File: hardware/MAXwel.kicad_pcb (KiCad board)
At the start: 2 copper layers, 85.1 x 87.2 mm, 155 parts, among them J1 Conn_02x05_Odd_Even, J2 Conn_02x12_Counter_Clockwise, J3 Barrel_Jack_Switch_Pin3Ring, SW1 SW_Push_Dual, SW10 SW_Wuerth_450301014042, SW11 SW_Wuerth_450301014042, SW12 SW_Wuerth_450301014042, SW13 SW_Wuerth_450301014042, SW2 SW_Push_Dual, SW3 SW_Push_Dual, SW4 SW_Push_Dual, SW5 SW_Wuerth_450301014042, SW6 SW_Wuerth_450301014042, SW7 SW_Wuerth_450301014042, SW8 SW_Wuerth_450301014042, SW9 SW_Push_DPDT, U1 D168K, U2 D168K, U3 D168K, U4 D168K, U5 EPM240T100, U6 AMS1117-3.3, X1 50.000, X2 14.756

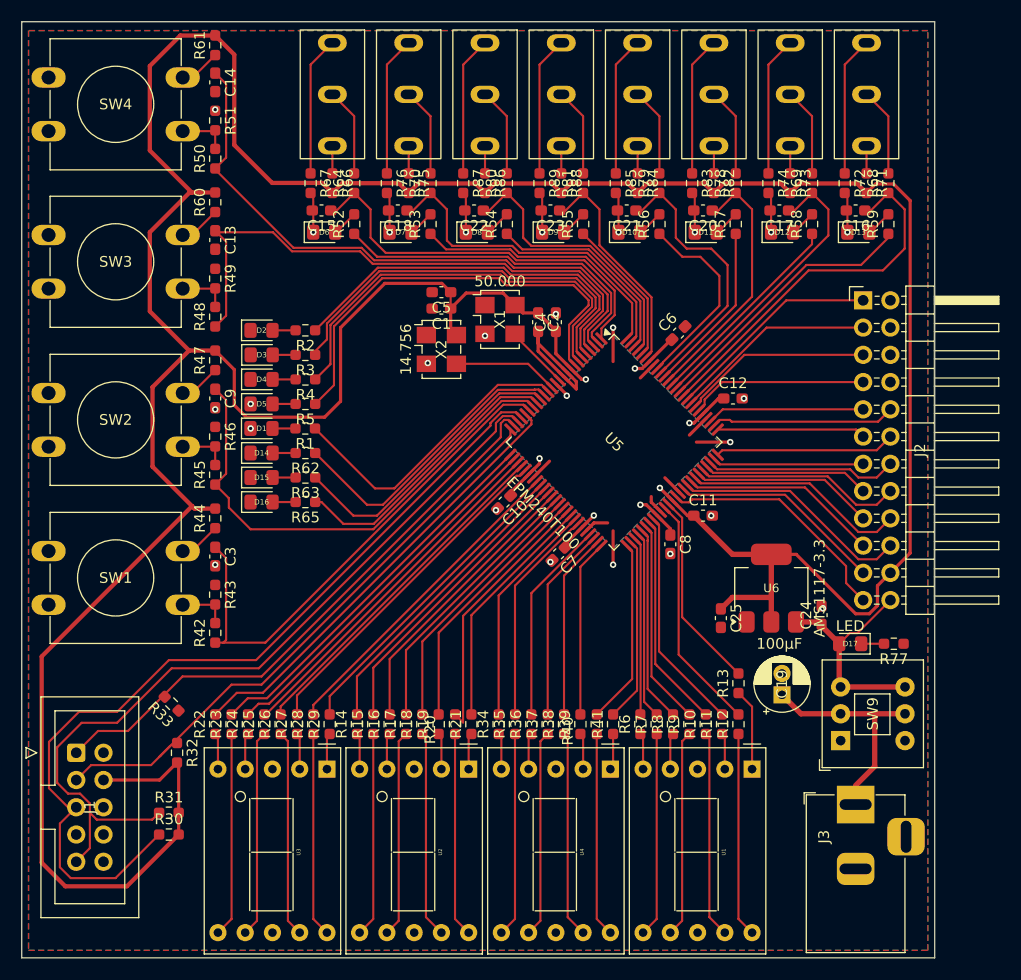
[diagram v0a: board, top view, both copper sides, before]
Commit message: squashing pcb layout
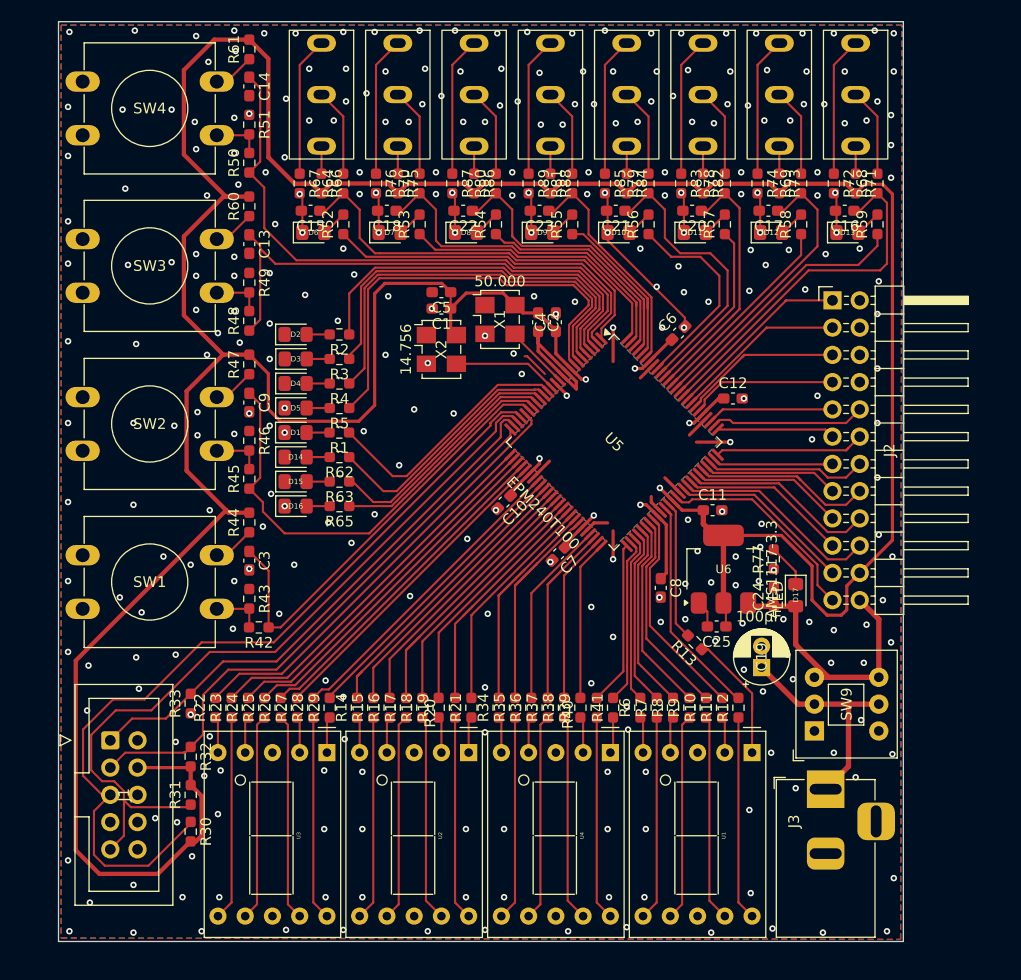
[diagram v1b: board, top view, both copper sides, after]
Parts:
- moved R77 13.7 mm to (174.2, 70.9), turned to 90 degrees
- moved D17 6.80 mm to (176.3, 74.2), turned to -90 degrees
- moved R13 5.57 mm to (166.9, 78.6), turned to 135 degrees
- moved U6 4.80 mm to (169.5, 71.8)
- moved C24 4.77 mm to (174.2, 74.3)
- moved C8 4.16 mm to (163.7, 73.5)
- moved R42 4.10 mm to (126.2, 77.2), turned to 180 degrees
- moved J1 3.38 mm to (112.4, 87.7)
- moved D2 3.20 mm to (129.7, 49.9)
- moved D3 3.20 mm to (129.7, 52.2)
- moved R1 3.20 mm to (133.7, 59.1)
- moved R2 3.20 mm to (133.8, 49.9)
- moved R3 3.20 mm to (133.8, 52.2)
- moved R4 3.20 mm to (133.8, 54.5)
- moved R5 3.20 mm to (133.8, 56.8)
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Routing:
- net GND: track 65.5 -> 83.5 mm, vias 25 -> 313
- net +3V3: track 371.0 -> 362.4 mm
- net Net-(U5-IO1_20): track 48.1 -> 41.0 mm
- net Net-(U1-E): track 7.61 -> 13.4 mm
- net +5V: track 21.6 -> 27.3 mm
- net Net-(U5-IO2_62/GCLK2): track 18.5 -> 13.0 mm
- net Net-(U5-IO1_18): track 26.6 -> 21.9 mm
- net Net-(U5-IO1_4): track 54.5 -> 49.8 mm
- net Net-(U5-IO1_17): track 27.4 -> 23.1 mm
- net Net-(U5-IO1_16): track 28.0 -> 23.7 mm
- net Net-(U5-IO1_15): track 28.3 -> 24.0 mm
- net Net-(J1-Pin_9): track 76.5 -> 72.5 mm
- net Net-(J1-Pin_5): track 82.3 -> 78.5 mm
- net Net-(J1-Pin_1): track 54.7 -> 51.0 mm
- net Net-(U5-IO1_19): track 46.8 -> 43.8 mm
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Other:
- board size 85.1 x 87.2 mm -> 78.7 x 85.7 mm
